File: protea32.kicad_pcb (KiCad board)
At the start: 2 copper layers, 68 x 66.5 mm, 146 parts, among them IC1 ESP32-D0WD-V3, J1 USB4215-03-A, J11 DC3RX19JA2, J2 676430910, J3 TTL, J4 D-SUB 9 Male, J5 0475710001, J6 Flash, Q1 2N7000, Q2 2N7000, Q3 2N7000, Q4 2N7000, Q5 2N7000, Q6 UMH3N, U10 W25Q32JVSIQ, U11 74HC4052D, U12 74HC4052D, U14 CH340C, U3 USBLC6-2SC6, U4 TS3USB221RSER, U5 NCP1117 3.3, U6 USBLC6-2SC6, U7 RP2040, U8 W25Q16JVSSIQ, U9 MAX232CSE+, Y2 ASE-12MHz, Y3 40MHz

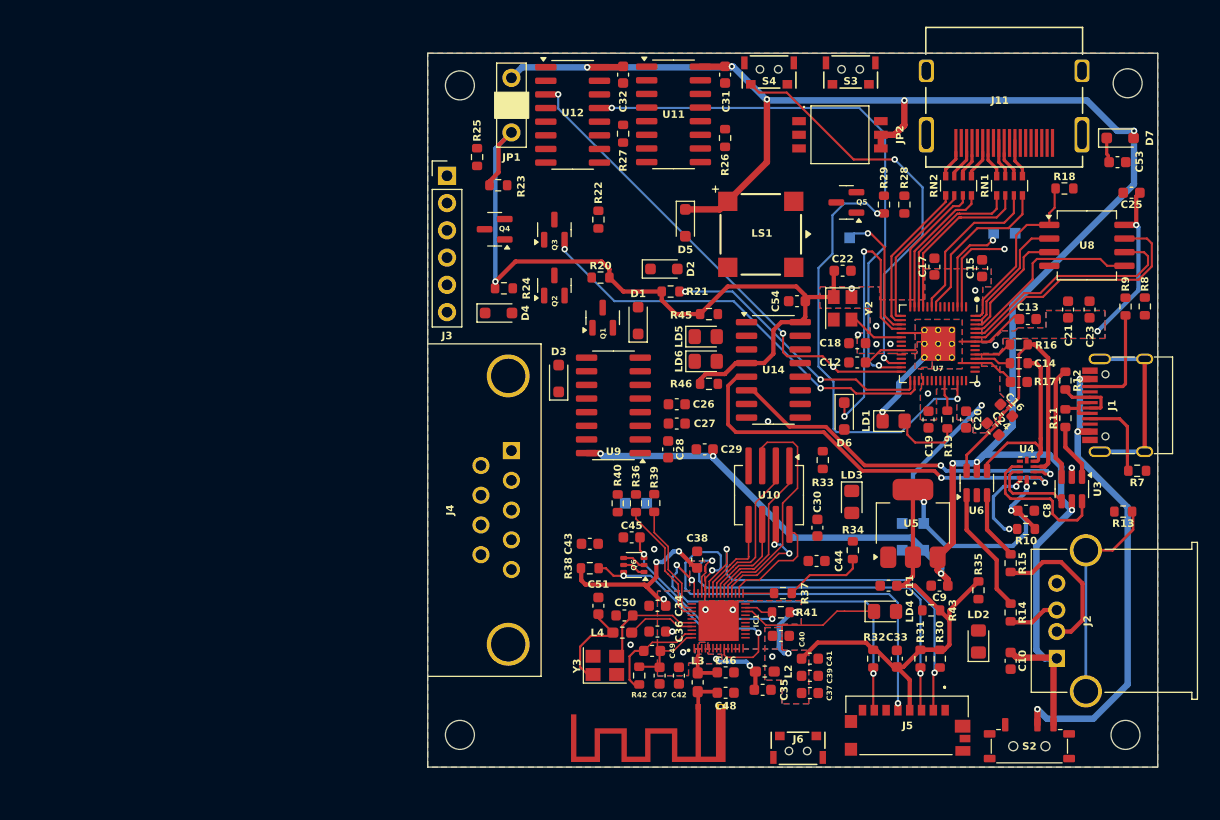
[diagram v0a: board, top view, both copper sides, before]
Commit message: Update protea32.kicad_pcb
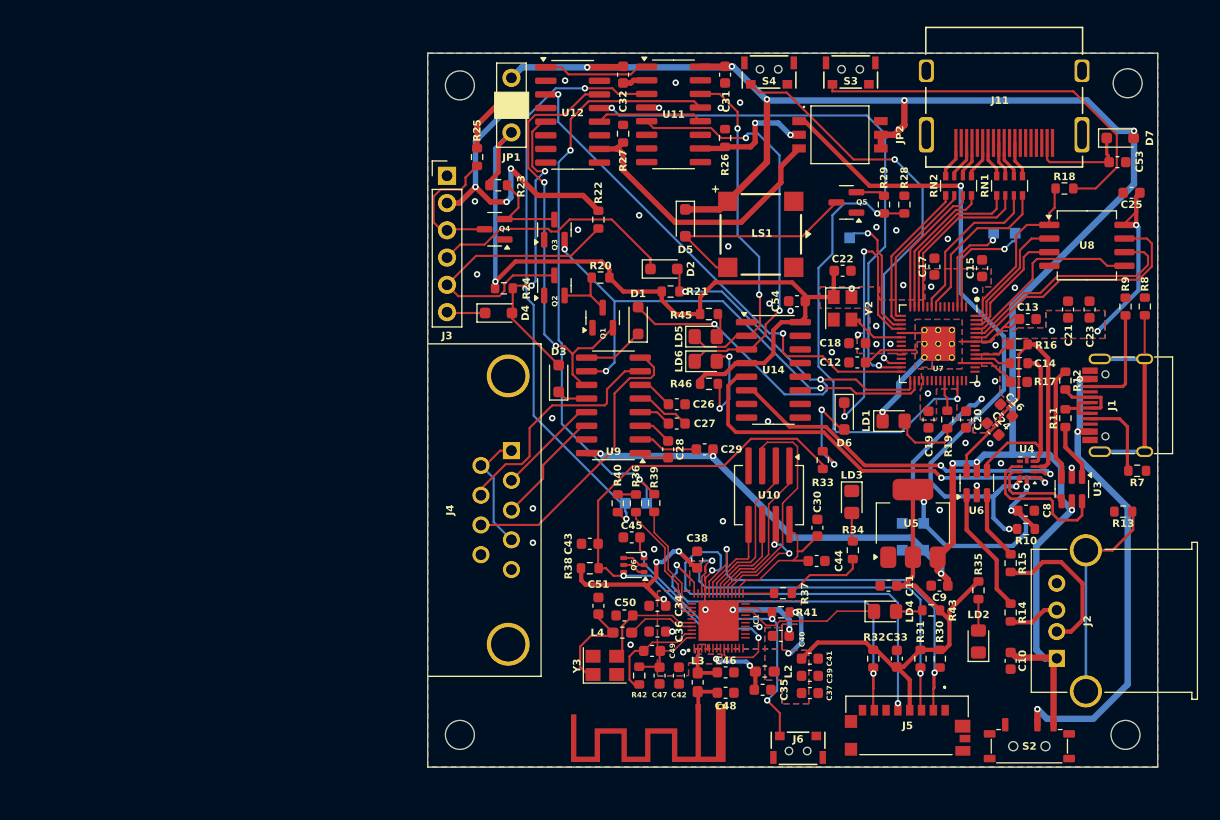
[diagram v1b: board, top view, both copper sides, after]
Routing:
- net /UMP_SW: track 7.43 -> 65.1 mm, vias 2 -> 3
- net /ESP_RXD: track 0.00 -> 55.8 mm, vias 0 -> 2
- net /ESP_TXD: track 0.00 -> 54.9 mm, vias 0 -> 2
- net /RS232_TX: track 0.00 -> 39.6 mm, vias 0 -> 2
- net /UT_RX: track 0.00 -> 38.6 mm, vias 0 -> 2
- net Net-(R18-Pad2): track 0.00 -> 36.7 mm
- net /RS232, TTL/VTTL: track 0.00 -> 34.9 mm, vias 0 -> 3
- net /UT_TX: track 0.00 -> 31.9 mm, vias 0 -> 2
- net /ESP_CHIP_PU: track 23.3 -> 54.4 mm
- net /RS232, TTL/TX_TTL: track 0.00 -> 27.9 mm
- net /RS232_RX: track 0.00 -> 27.5 mm, vias 0 -> 2
- net /RS232, TTL/RTS_IN: track 0.00 -> 26.9 mm
- net /M2_SW: track 0.00 -> 26.9 mm
- net /RP_GPIO18: track 25.5 -> 50.3 mm, vias 2 -> 3
- net /RS232, TTL/CTS_TTL: track 0.00 -> 23.1 mm
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
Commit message: Routing WIP
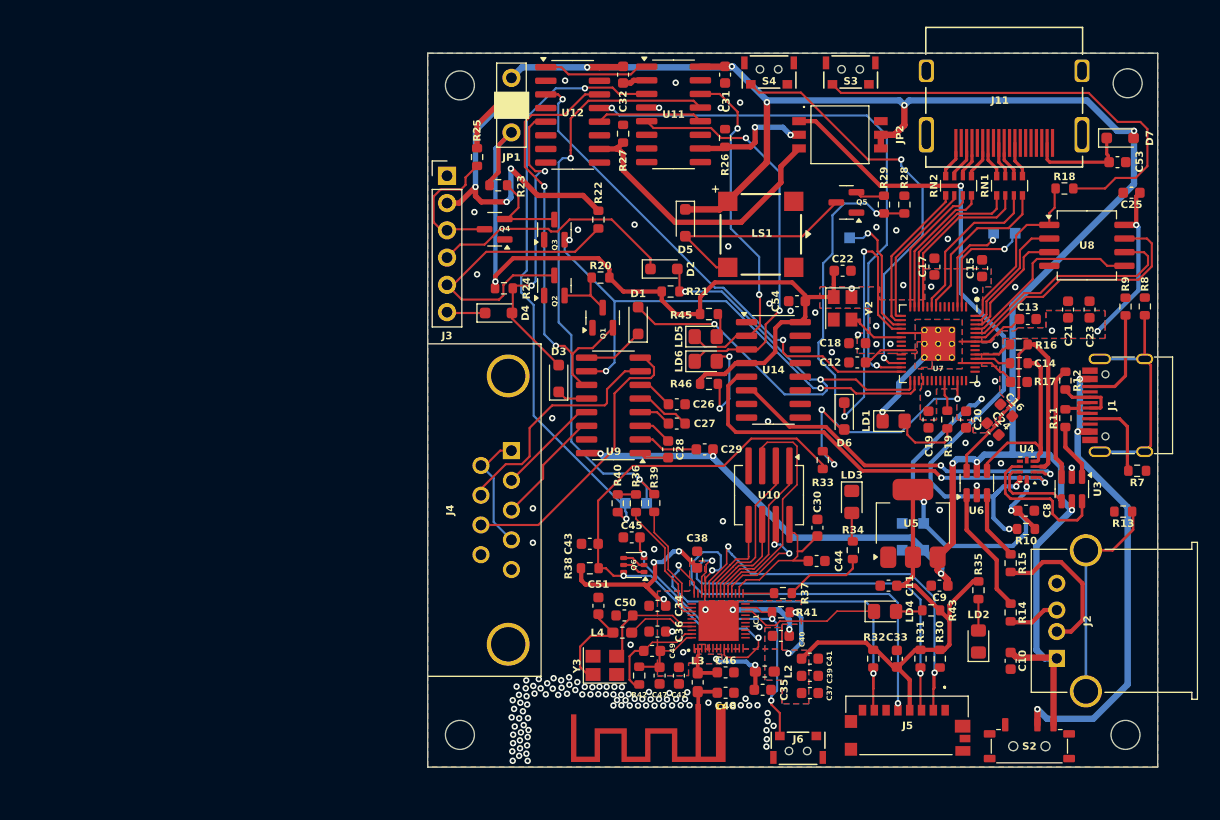
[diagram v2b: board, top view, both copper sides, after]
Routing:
- net Net-(R18-Pad2): track 36.7 -> 42.3 mm
- net Net-(U7-VREG_VOUT): track 18.5 -> 17.0 mm
- net /ESP_GPIO18: track 41.1 -> 39.6 mm
- net /RS232, TTL/VTTL: track 34.9 -> 36.0 mm
- net /UT_RX: track 38.6 -> 37.6 mm
- net /ESP_RXD: track 55.8 -> 56.8 mm
- net /RS232_RX: track 27.5 -> 28.5 mm
- net +3V3: track 195.9 -> 195.2 mm
- net /RP_GPIO19: track 48.8 -> 49.4 mm
- net /M1_SW: track 10.7 -> 10.2 mm
- net /RP_GPIO0: track 10.9 -> 10.3 mm
- net /UT_TX: track 31.9 -> 32.4 mm
- net GND: vias 35 -> 127

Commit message: Cleanup WIP
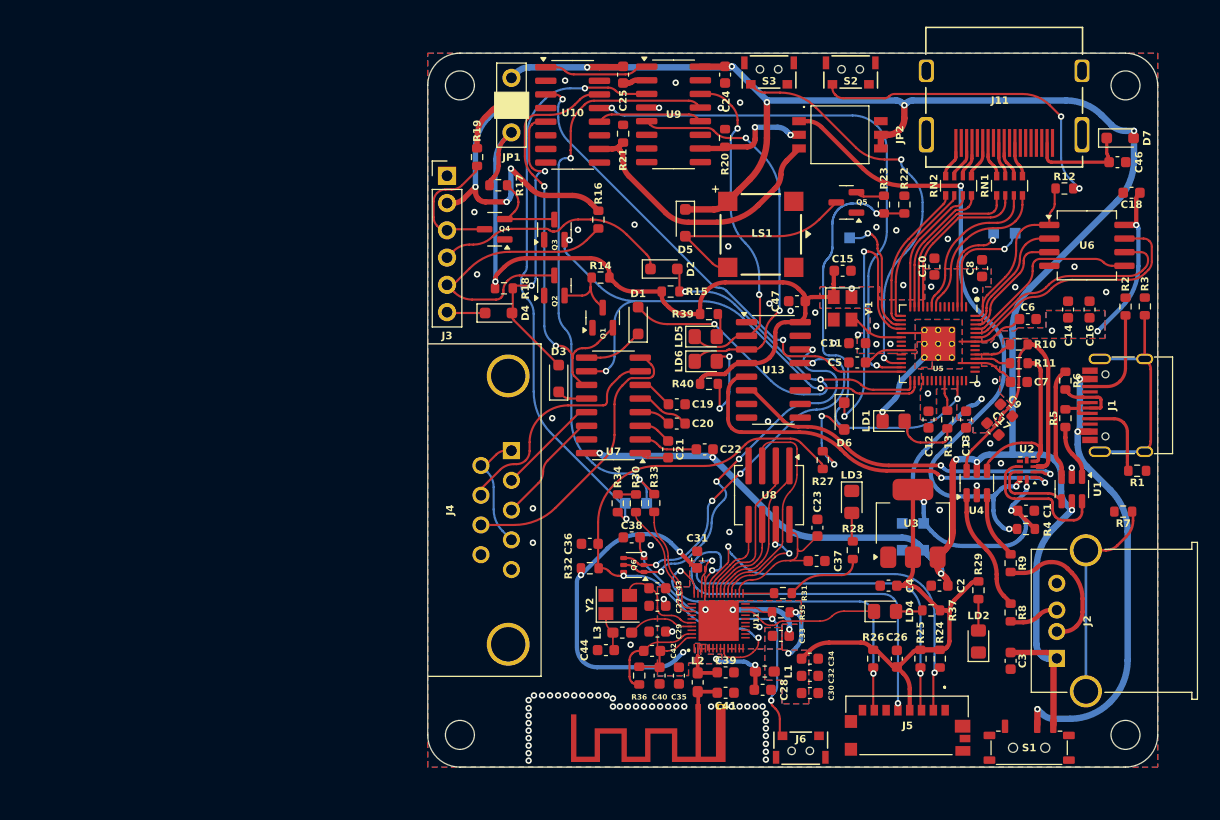
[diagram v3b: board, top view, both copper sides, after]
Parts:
- moved Y2 5.80 mm to (182.4, 113.8)
- moved C44 4.18 mm to (181.3, 118.1), turned to 180 degrees
- moved C43 3.98 mm to (186.1, 112.3), turned to 0 degrees
- moved H2 0.28 mm to (229.7, 65.5)
- moved J6 0.25 mm to (199.4, 127.5)
- moved S1 0.15 mm to (220.7, 127.2)
- renumbered AE2 to AE1, C8 to C1, C17 to C10, C18 to C11, C19 to C12, C20 to C13, C21 to C14, C22 to C15, C23 to C16, C24 to C17, C25 to C18, C26 to C19, C9 to C2, C27 to C20, C28 to C21, C29 to C22, C30 to C23, C31 to C24, C32 to C25, C33 to C26, C34 to C27, C35 to C28, C36 to C29, C10 to C3, C37 to C30, C38 to C31, C39 to C32, C40 to C33, C41 to C34, C42 to C35, C43 to C36, C44 to C37, C45 to C38, C46 to C39, C11 to C4, C47 to C40, C48 to C41, C49 to C42, C50 to C43, C51 to C44, C53 to C46, C54 to C47, C12 to C5, C13 to C6, C14 to C7, C15 to C8, C16 to C9, L2 to L1, L3 to L2, L4 to L3, R7 to R1, R16 to R10, R17 to R11, R18 to R12, R19 to R13, R20 to R14, R21 to R15, R22 to R16, R23 to R17, R24 to R18, R25 to R19, R8 to R2, R26 to R20, R27 to R21, R28 to R22, R29 to R23, R30 to R24, R31 to R25, R32 to R26, R33 to R27, R34 to R28, R35 to R29, R9 to R3, R36 to R30, R37 to R31, R38 to R32, R39 to R33, R40 to R34, R41 to R35, R42 to R36, R43 to R37, R45 to R39, R10 to R4, R46 to R40, R11 to R5, R12 to R6, R13 to R7, R14 to R8, R15 to R9, S2 to S1, S3 to S2, S4 to S3, U3 to U1, U12 to U10, IC1 to U11, U14 to U13, U4 to U2, U5 to U3, U6 to U4, U7 to U5, U8 to U6, U9 to U7, U10 to U8, U11 to U9, Y2 to Y1, Y3 to Y2
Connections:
- U13 pad 13: /UT_DTR -> /ESP_DTR
- U13 pad 14: /UT_RTS -> /ESP_RTS
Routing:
- net /ESP_RTS: track 2.17 -> 36.0 mm, vias 0 -> 4
- net /ESP_DTR: track 2.17 -> 33.6 mm, vias 0 -> 4
- net Net-(R12-Pad2): track 42.3 -> 30.2 mm, vias 0 -> 2
- net VBUS: track 219.1 -> 213.4 mm
- net +3V3: track 195.2 -> 200.8 mm
- net Net-(C44-Pad1): track 8.34 -> 3.35 mm
- net /ESP_GPIO19: track 36.3 -> 33.4 mm
- net /ESP32/XTAL_N: track 10.2 -> 7.73 mm
- net /UT_TX: track 32.4 -> 30.2 mm
- net /ESP_GPIO5: track 39.1 -> 37.0 mm
- net /UMP_SW: track 65.1 -> 62.9 mm
- net /RS232, TTL/VTTL: track 36.0 -> 34.1 mm
- net /ESP_CHIP_PU: track 54.0 -> 52.2 mm
- net /RS232, TTL/CTS_IN: track 21.7 -> 20.3 mm
- net /RP_GPIO17: track 46.8 -> 45.4 mm
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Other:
- outline, holes or cut-outs redrawn

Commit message: HW 1.00
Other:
- board text added: "${NAME}"
- board text added: "HW ${VERSION}"
- board text added: "RH1.TECH"

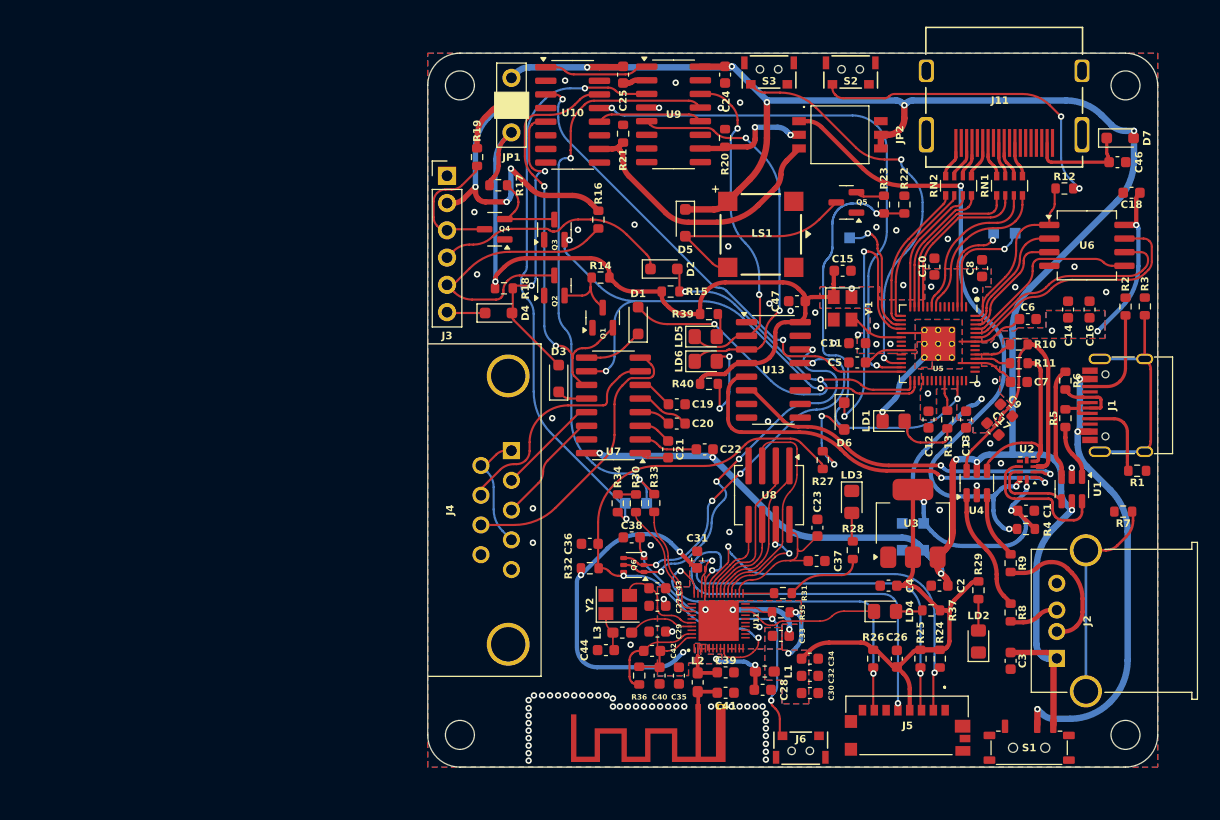
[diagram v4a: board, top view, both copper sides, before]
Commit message: HW 1.01
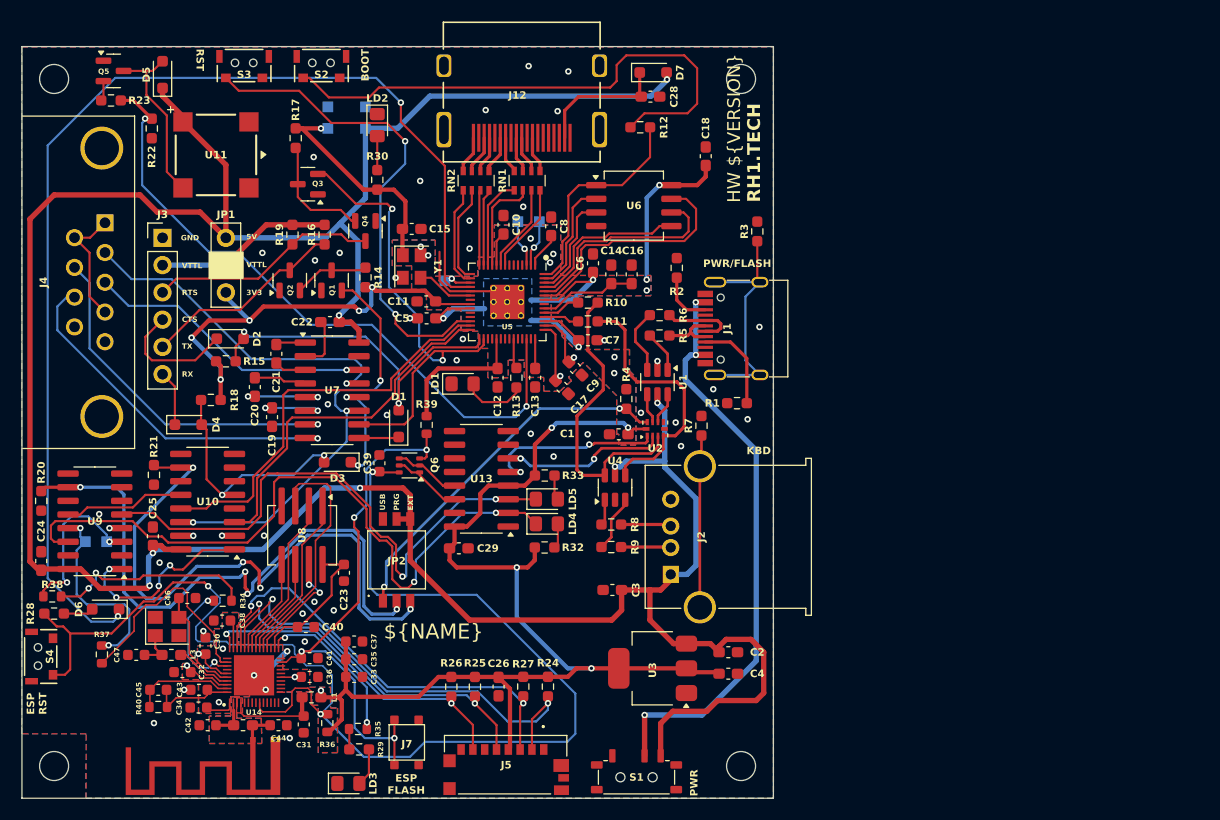
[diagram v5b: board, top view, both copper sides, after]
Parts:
- removed C27: 1u, FRANK:Capacitor (0603, S)
- removed the C28 at (195.9, 121.8)
- removed LD6: Orange, FRANK:LED (0805)
- removed LS1: CMT-7525-80-SMT-TR, FRANK:CMT752580SMTTR
- removed R31: 0R, FRANK:Resistor (0603, S)
- removed TP1: Defaults, FRANK:Test Point (1mm x 1)
- added C45: 3.3n, FRANK:Capacitor (0603, S), F.Cu at (139.6, 121.8)
- added C46: 12p, FRANK:Capacitor (0603, S), F.Cu at (142.3, 113.2)
- added J11: ~, FRANK:Test Points (1mm x 2), B.Cu at (158.9, 67.5)
- added R38: 330R, FRANK:Resistor (0603, S), F.Cu at (129.7, 113.1)
- added S4: ESP RST, FRANK:TACT-SIDE-4623, F.Cu at (128.4, 118.7)
- added U14: ESP32-D0WD-V3, FRANK:QFN35P500X500X90-49N-D, F.Cu at (148.5, 120.5)
- C1, C10, C11, C12, C13, C14, C15, C16, C17, C18, C19, C2, C20, C21, C22, C24, C25, C26, C3, C4, C5, C6, C7, C8, C9: footprint FRANK:Capacitor (0603, S) -> FRANK:Capacitor (0603)
- C28: renamed from C46; footprint FRANK:Capacitor (0603, S) -> FRANK:Capacitor (0603)
- C29: value 100p -> 100n; footprint FRANK:Capacitor (0603, S) -> FRANK:Capacitor (0603)
- C30: value 100n -> 1u
- C32: value 10u -> 100p
- C34: value 1u -> 100n
- C35: value 100n -> 10u
- C36, C38: value 1n -> 100n
- C39: value 1.5pF -> 1n
- C40: value 10n -> 1u
- C41: value 2.4pF -> 1n
- C42: value 3.3n -> 1.5pF
- C43: value 12p -> 10n
- C44: value 12p -> 2.4pF
- C47: value 100n -> 12p
- J6: value Flash -> Defaults; footprint FRANK:TACT-SIDE-4623 -> FRANK:Test Point (1mm x 1); moved to B.Cu
- J7: value ~ -> Flash; footprint FRANK:Test Points (1mm x 2) -> FRANK:Button (SMD, 3x3mm, 1-1); moved to F.Cu
- LD4: value Blue -> Orange
- R1, R10, R11, R12, R13, R14, R15, R16, R17, R18, R19, R2, R20, R21, R22, R23, R24, R25, R26, R3, R4, R5, R6, R7, R8, R9: footprint FRANK:Resistor (0603, S) -> FRANK:Resistor (0603)
- R27: value 200R -> 10K; footprint FRANK:Resistor (0603, S) -> FRANK:Resistor (0603)
- R28: value 470R -> 200R; footprint FRANK:Resistor (0603, S) -> FRANK:Resistor (0603)
- R29: value 1K -> 470R; footprint FRANK:Resistor (0603, S) -> FRANK:Resistor (0603)
- R30: value 499R -> 1K; footprint FRANK:Resistor (0603, S) -> FRANK:Resistor (0603)
- R32: value 10K -> 1.5K; footprint FRANK:Resistor (0603, S) -> FRANK:Resistor (0603)
- R33: value 330R -> 1.5K; footprint FRANK:Resistor (0603, S) -> FRANK:Resistor (0603)
- R34: value 330R -> 499R
- R35: value 10K -> 0R
- R36: value 20K -> 10K
- R37: value 5.1K -> 330R
- R39: value 1.5K -> 10K
- R40: value 1.5K -> 20K
- U11: value ESP32-D0WD-V3 -> CMT-7525-80-SMT-TR; footprint FRANK:QFN35P500X500X90-49N-D -> FRANK:CMT752580SMTTR
- moved H3 99.8 mm to (129.9, 128.9)
- moved J8 91.3 mm to (132.8, 108.0), turned to -90 degrees
- moved C24 78.2 mm to (128.7, 109.8), turned to -90 degrees
- moved R37 77.4 mm to (134.3, 118.5), turned to -90 degrees
- moved R28 74.6 mm to (129.9, 114.7), turned to 0 degrees
- moved LD2 73.8 mm to (160.0, 69.2), turned to -90 degrees
- moved R23 72.7 mm to (135.2, 66.9), turned to 0 degrees
- moved R20 72.1 mm to (128.7, 104.2), turned to 90 degrees
- moved D6 71.1 mm to (134.7, 114.3), turned to 180 degrees
- moved R22 70.5 mm to (139.0, 69.5), turned to 90 degrees
- moved C47 69.8 mm to (137.6, 118.5)
- moved Q5 69.4 mm to (135.4, 64.2), turned to 0 degrees
- moved J10 67.6 mm to (155.4, 67.5), turned to 180 degrees
- moved U9 65.9 mm to (133.7, 106.1), turned to 180 degrees
- moved U11 63.9 mm to (145.0, 72.0), turned to 0 degrees
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- renumbered J11 to J12
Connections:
- C31 pad 1: +3V3 -> +3.3VP
- C36 pad 1: /ESP_CHIP_PU -> +3V3
- C37 pad 1: /VDD_SDIO -> +3V3
- C38 pad 1: /ESP_GPIO0 -> +3V3
- C39 pad 1: /ESP32/LNA_IN -> /ESP_CHIP_PU
- C40 pad 1: /ESP32/CAP1 -> /VDD_SDIO
- C41 pad 1: /ESP32/ANT -> /ESP_GPIO0
- C42 pad 1: /ESP32/CAP1 -> /ESP32/LNA_IN
- C42 pad 2: /ESP32/CAP2 -> GND
- C43 pad 1: /ESP32/XTAL_N -> /ESP32/CAP1
- C44 pad 1: Net-(C44-Pad1) -> /ESP32/ANT
- C47 pad 1: +3V3 -> Net-(C47-Pad1)
- J10 pad 2: VBUS -> +3V3
- J6 pad 1: GND -> /RP_GPIO14
- J7 pad 1: /ESP_RXD -> GND
- J7 pad 2: /ESP_TXD -> /ESP_GPIO0
- J8 pad 1: /RP_GPIO0 -> /ESP_RXD
- J8 pad 2: /RP_GPIO1 -> /ESP_TXD
- J9 pad 1: GND -> /RP_GPIO0
- J9 pad 2: +3V3 -> /RP_GPIO1
- L3 pad 2: Net-(C44-Pad1) -> Net-(C47-Pad1)
- LD4 pad 1: /ESP_GPIO2 -> /UT_TX
- LD5 pad 1: /UT_TX -> /UT_RX
- R25 pad 1: /ESP_GPIO23 -> /ESP_GPIO18
- R27 pad 1: /ESP_CHIP_PU -> /ESP_GPIO23
- R27 pad 2: Net-(D6-A) -> +3V3
- R28 pad 1: /ESP_GPIO16 -> /ESP_CHIP_PU
- R28 pad 2: Net-(LD3-A) -> Net-(D6-A)
- R29 pad 1: Net-(LD2-A) -> /ESP_GPIO16
- R29 pad 2: +3V3 -> Net-(LD3-A)
- R30 pad 1: Net-(U11-U0TXD) -> Net-(LD2-A)
- R30 pad 2: /ESP_U0TXD -> +3V3
- R32 pad 1: /ESP_CHIP_PU -> Net-(LD4-A)
- R33 pad 1: /ESP_RXD -> +3V3
- R33 pad 2: /ESP_U0RXD -> Net-(LD5-A)
- R34 pad 1: /ESP_TXD -> Net-(U14-U0TXD)
- R35 pad 1: /ESP_GPIO0 -> Net-(U14-GPIO16)
- R35 pad 2: +3V3 -> /ESP_GPIO16
- R36 pad 1: /ESP32/CAP2 -> /ESP_CHIP_PU
- R36 pad 2: /ESP32/CAP1 -> +3V3
- R37 pad 1: +3V3 -> /ESP_RXD
- R37 pad 2: Net-(LD4-A) -> /ESP_U0RXD
- R39 pad 1: Net-(LD5-A) -> /ESP_GPIO0
- R40 pad 1: +3V3 -> /ESP32/CAP2
- R40 pad 2: Net-(LD6-A) -> /ESP32/CAP1
- U11 pad 1: +3V3 -> VBUS
- U11 pad 2: /ESP32/LNA_IN -> Net-(D5-A)
- U11 pad 3: +3.3VP -> unconnected-(U11-DUMMY_1-Pad3)
- U11 pad 4: +3.3VP -> unconnected-(U11-DUMMY_2-Pad4)
- Y2 pad 1: Net-(C44-Pad1) -> Net-(C47-Pad1)
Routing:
- net /RP_GPIO15: track 26.6 -> 106.7 mm
- net /ESP_CHIP_PU: track 52.2 -> 124.4 mm, vias 2 -> 3
- net VBUS: track 213.4 -> 272.0 mm, vias 11 -> 7
- net /M1_SW: track 10.0 -> 56.4 mm, vias 2 -> 4
- net /ESP_TXD: track 54.5 -> 14.3 mm
- net /ESP_RXD: track 55.7 -> 16.8 mm
- net +3V3: track 200.8 -> 237.1 mm, vias 27 -> 28
- net /UT_TX: track 30.2 -> 65.0 mm
- net /M2_SW: track 26.0 -> 55.9 mm, vias 0 -> 4
- net /ESP_RTS: track 36.0 -> 6.60 mm, vias 4 -> 0
- net /UMP_SW: track 62.9 -> 33.8 mm, vias 3 -> 2
- net /ESP_DTR: track 33.6 -> 6.20 mm, vias 4 -> 0
- net /RS232, TTL/TX_IN: track 8.98 -> 30.7 mm, vias 0 -> 1
- net /UT_D+: track 37.4 -> 16.2 mm
- net Net-(R12-Pad2): track 30.2 -> 50.9 mm, vias 2 -> 0
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- removed copper zone on B.Cu, net +3.3VP
- removed copper zone on F.Cu, net Net-(U5-VREG_VOUT)
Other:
- board size 68 x 66.5 mm -> 70 x 70 mm
- board text added: "3V3"
- board text added: "5V"
- board text added: "BOOT"
- board text added: "CTS"
- board text added: "ESP FLASH"
- board text added: "ESP RST"
- board text added: "EXT"
- board text added: "GND"
- board text added: "GPIO0"
- board text added: "GPIO1"
- board text added: "GPIO14"
- board text added: "KBD"
- board text added: "PRG"
- board text added: "PWR"
- board text added: "PWR/FLASH"
- board text added: "RST"
- board text added: "RTS"
- board text added: "RX"
- board text added: "TX"
- board text added: "USB"
- board text added: "VTTL"
